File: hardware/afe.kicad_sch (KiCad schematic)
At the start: 6 parts, among them U2 LTC6813-1, U3 BQ76200PW

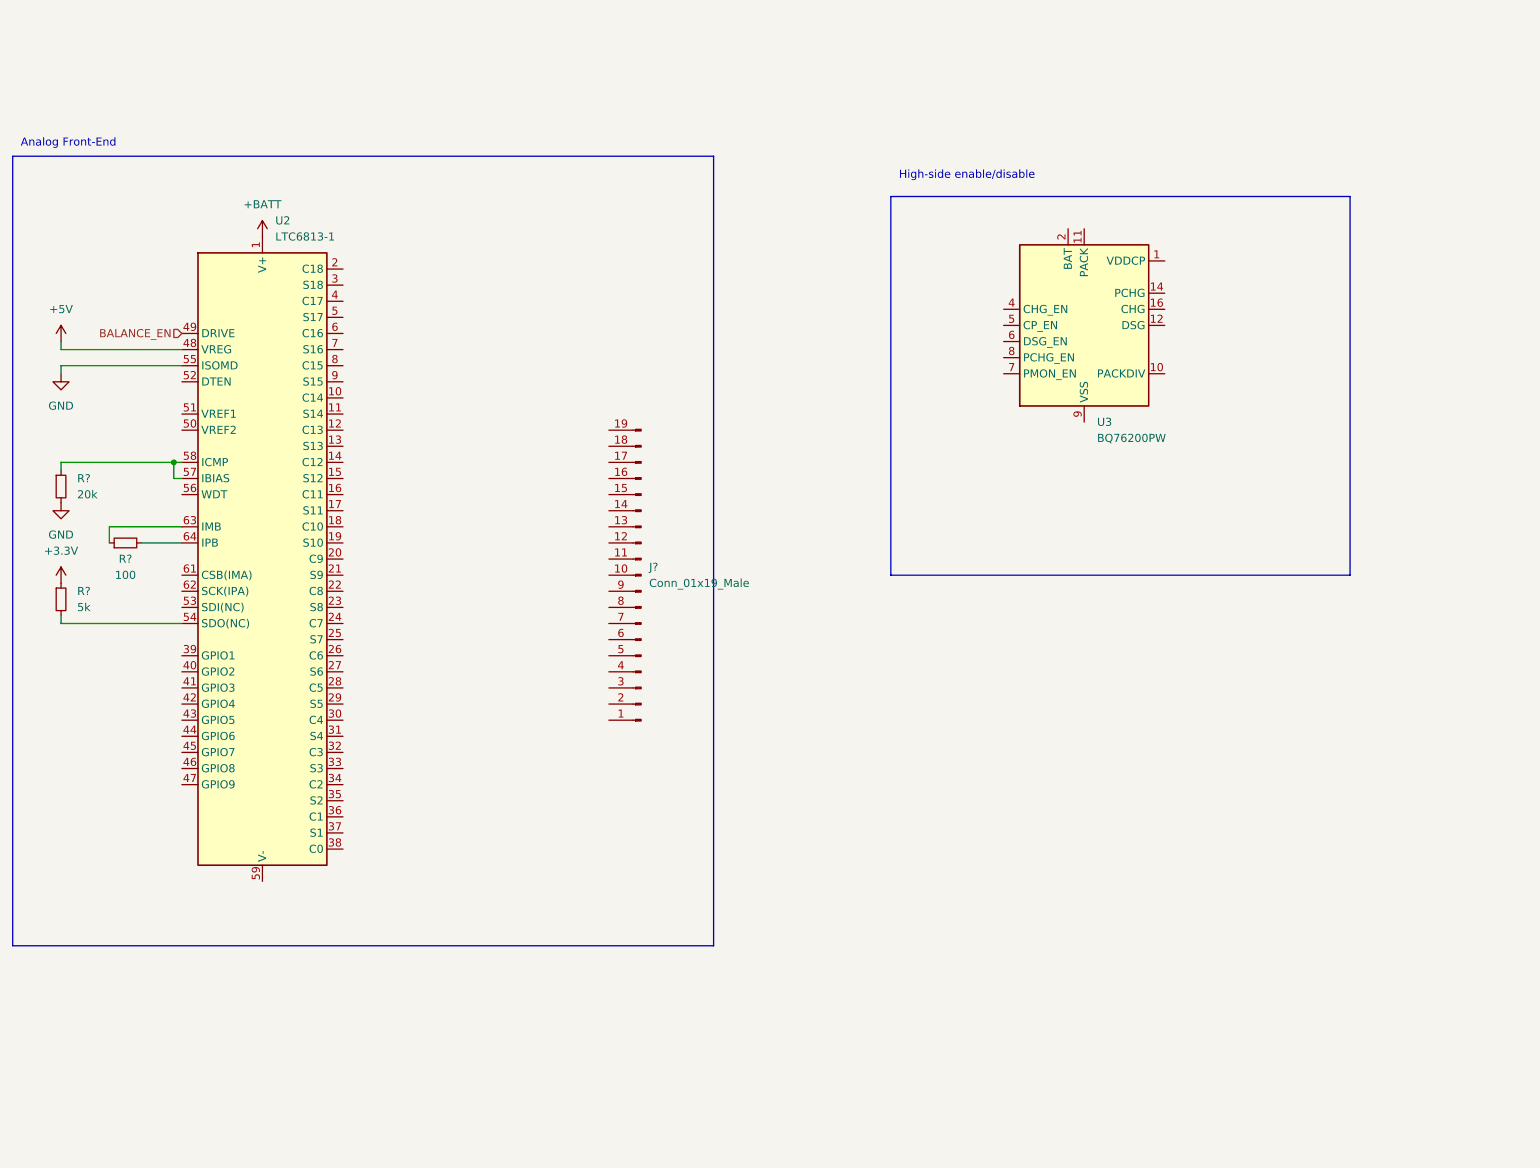
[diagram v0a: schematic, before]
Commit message: Balance frontend
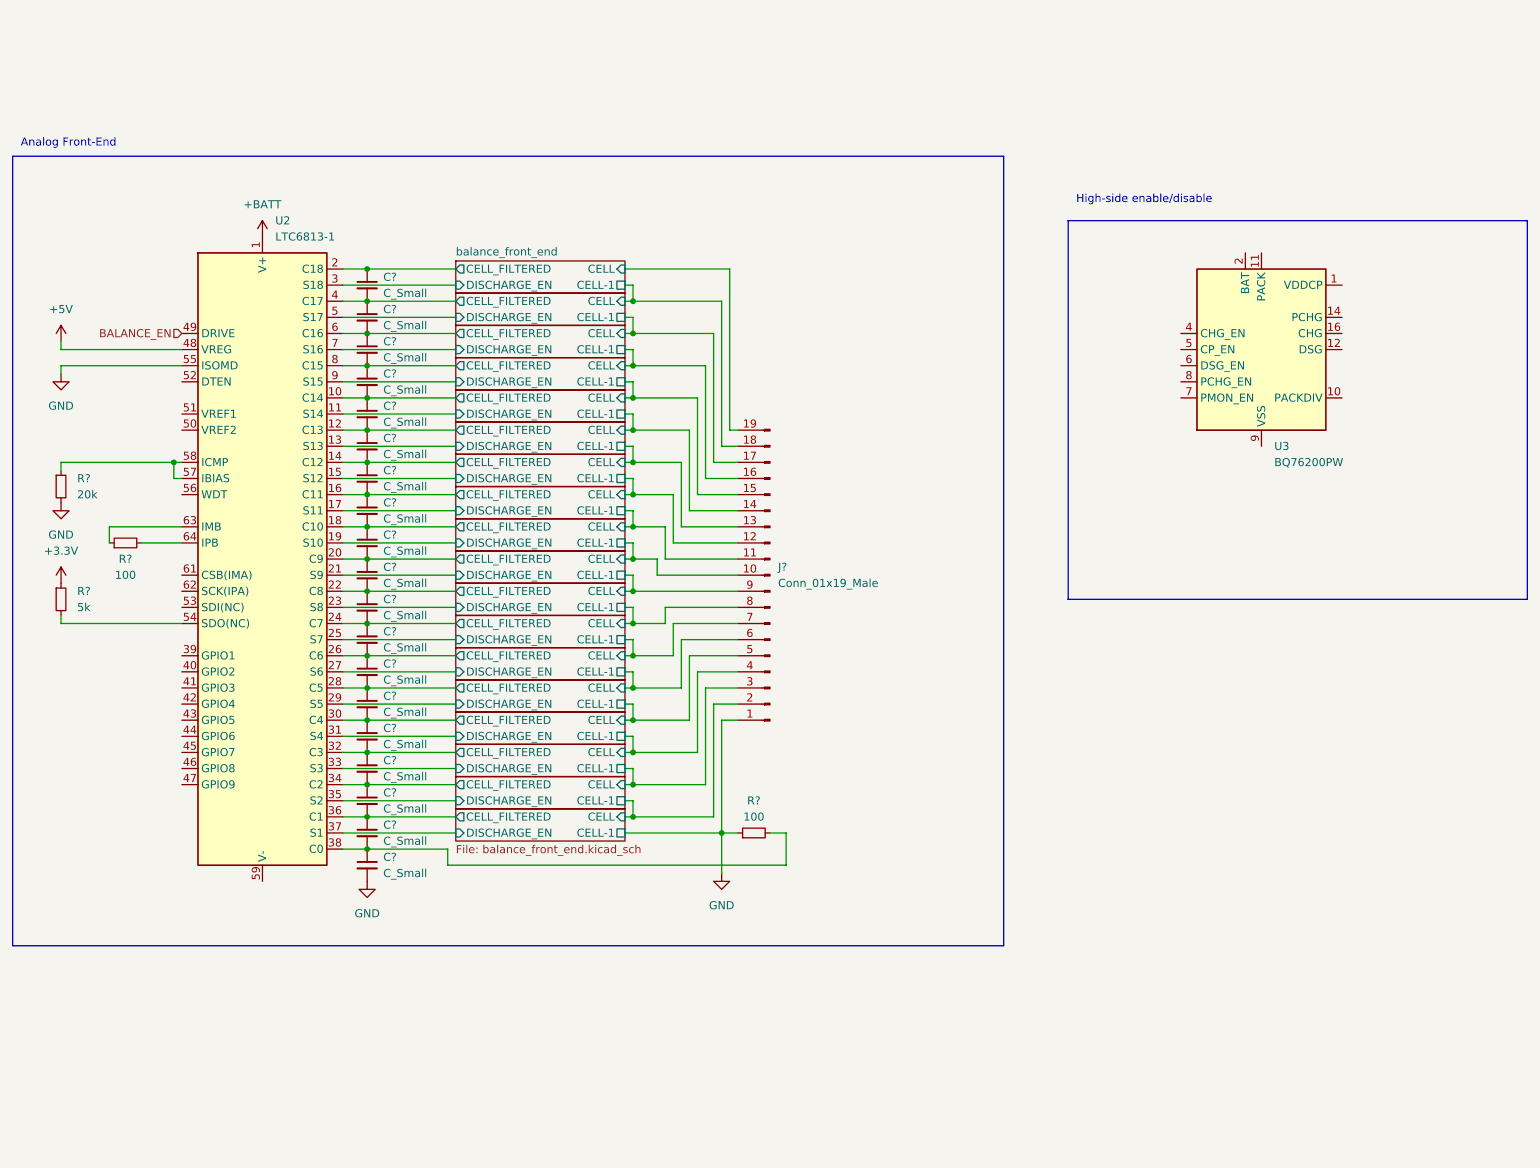
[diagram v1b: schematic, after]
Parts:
- added C? (x19): C_Small, symbol Device:C_Small
- added R?: 100, symbol Device:R_Small
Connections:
- net GND: now also J?.1 (Pin_1), C?.2, R?.1
- net balance_front_end6/CELL_FILTERED: now reaches U2.10 (C14)
- net balance_front_end6/CELL_FILTERED: now also C?.1, C?.2
- net balance_front_end6/DISCHARGE_EN: now reaches U2.11 (S14)
- net balance_front_end5/CELL_FILTERED: now reaches U2.12 (C13)
- net balance_front_end5/CELL_FILTERED: now also C?.1, C?.2
- net balance_front_end5/DISCHARGE_EN: now reaches U2.13 (S13)
- net balance_front_end4/CELL_FILTERED: now reaches U2.14 (C12)
- net balance_front_end4/CELL_FILTERED: now also C?.1, C?.2
- net balance_front_end4/DISCHARGE_EN: now reaches U2.15 (S12)
- net balance_front_end10/CELL_FILTERED: now reaches U2.16 (C11)
- net balance_front_end10/CELL_FILTERED: now also C?.1, C?.2
- net balance_front_end10/DISCHARGE_EN: now reaches U2.17 (S11)
- net balance_front_end9/CELL_FILTERED: now reaches U2.18 (C10)
- net balance_front_end9/CELL_FILTERED: now also C?.1, C?.2
- net balance_front_end9/DISCHARGE_EN: now reaches U2.19 (S10)
- net balance_front_end/CELL_FILTERED: now reaches U2.2 (C18)
- net balance_front_end/CELL_FILTERED: now also C?.1
- net balance_front_end7/CELL_FILTERED: now reaches U2.20 (C9)
- net balance_front_end7/CELL_FILTERED: now also C?.1, C?.2
- net balance_front_end7/DISCHARGE_EN: now reaches U2.21 (S9)
- net balance_front_end11/CELL_FILTERED: now reaches U2.22 (C8)
- net balance_front_end11/CELL_FILTERED: now also C?.1, C?.2
- net balance_front_end11/DISCHARGE_EN: now reaches U2.23 (S8)
- net balance_front_end12/CELL_FILTERED: now reaches U2.24 (C7)
- net balance_front_end12/CELL_FILTERED: now also C?.1, C?.2
- net balance_front_end12/DISCHARGE_EN: now reaches U2.25 (S7)
- net balance_front_end8/CELL_FILTERED: now reaches U2.26 (C6)
- net balance_front_end8/CELL_FILTERED: now also C?.1, C?.2
- net balance_front_end8/DISCHARGE_EN: now reaches U2.27 (S6)
- net balance_front_end13/CELL_FILTERED: now reaches U2.28 (C5)
- net balance_front_end13/CELL_FILTERED: now also C?.1, C?.2
- net balance_front_end13/DISCHARGE_EN: now reaches U2.29 (S5)
- net balance_front_end/DISCHARGE_EN: now reaches U2.3 (S18)
- net balance_front_end16/CELL_FILTERED: now reaches U2.30 (C4)
- net balance_front_end16/CELL_FILTERED: now also C?.1, C?.2
- net balance_front_end16/DISCHARGE_EN: now reaches U2.31 (S4)
- net balance_front_end14/CELL_FILTERED: now reaches U2.32 (C3)
- net balance_front_end14/CELL_FILTERED: now also C?.1, C?.2
- net balance_front_end14/DISCHARGE_EN: now reaches U2.33 (S3)
- net balance_front_end15/CELL_FILTERED: now reaches U2.34 (C2)
- net balance_front_end15/CELL_FILTERED: now also C?.1, C?.2
- net balance_front_end15/DISCHARGE_EN: now reaches U2.35 (S2)
- net balance_front_end17/CELL_FILTERED: now reaches U2.36 (C1)
- net balance_front_end17/CELL_FILTERED: now also C?.1, C?.2
- net balance_front_end17/DISCHARGE_EN: now reaches U2.37 (S1)
- net at U2.38 (C0): now also C?.1, C?.2, R?.2
- net balance_front_end1/CELL_FILTERED: now reaches U2.4 (C17)
- net balance_front_end1/CELL_FILTERED: now also C?.1, C?.2
- net balance_front_end1/DISCHARGE_EN: now reaches U2.5 (S17)
- net balance_front_end2/CELL_FILTERED: now reaches U2.6 (C16)
- net balance_front_end2/CELL_FILTERED: now also C?.1, C?.2
- net balance_front_end2/DISCHARGE_EN: now reaches U2.7 (S16)
- net balance_front_end3/CELL_FILTERED: now reaches U2.8 (C15)
- net balance_front_end3/CELL_FILTERED: now also C?.1, C?.2
- net balance_front_end3/DISCHARGE_EN: now reaches U2.9 (S15)
- net balance_front_end7/CELL: now reaches J?.10 (Pin_10)
- net balance_front_end10/CELL-1: now reaches J?.11 (Pin_11)
- net balance_front_end10/CELL: now reaches J?.12 (Pin_12)
- net balance_front_end4/CELL: now reaches J?.13 (Pin_13)
- net balance_front_end5/CELL: now reaches J?.14 (Pin_14)
- net balance_front_end3/CELL-1: now reaches J?.15 (Pin_15)
- net balance_front_end2/CELL-1: now reaches J?.16 (Pin_16)
- net balance_front_end1/CELL-1: now reaches J?.17 (Pin_17)
- net balance_front_end/CELL-1: now reaches J?.18 (Pin_18)
- net balance_front_end/CELL: now reaches J?.19 (Pin_19)
- net balance_front_end15/CELL-1: now reaches J?.2 (Pin_2)
- net balance_front_end14/CELL-1: now reaches J?.3 (Pin_3)
- net balance_front_end14/CELL: now reaches J?.4 (Pin_4)
- net balance_front_end13/CELL-1: now reaches J?.5 (Pin_5)
- net balance_front_end13/CELL: now reaches J?.6 (Pin_6)
- net balance_front_end12/CELL-1: now reaches J?.7 (Pin_7)
- net balance_front_end11/CELL-1: now reaches J?.8 (Pin_8)
- net balance_front_end11/CELL: now reaches J?.9 (Pin_9)
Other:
- added sheet balance_front_end (balance_front_end.kicad_sch)
- added sheet balance_front_end1 (balance_front_end.kicad_sch)
- added sheet balance_front_end10 (balance_front_end.kicad_sch)
- added sheet balance_front_end11 (balance_front_end.kicad_sch)
- added sheet balance_front_end12 (balance_front_end.kicad_sch)
- added sheet balance_front_end13 (balance_front_end.kicad_sch)
- added sheet balance_front_end14 (balance_front_end.kicad_sch)
- added sheet balance_front_end15 (balance_front_end.kicad_sch)
- added sheet balance_front_end16 (balance_front_end.kicad_sch)
- added sheet balance_front_end17 (balance_front_end.kicad_sch)
- added sheet balance_front_end2 (balance_front_end.kicad_sch)
- added sheet balance_front_end3 (balance_front_end.kicad_sch)
- added sheet balance_front_end4 (balance_front_end.kicad_sch)
- added sheet balance_front_end5 (balance_front_end.kicad_sch)
- added sheet balance_front_end6 (balance_front_end.kicad_sch)
- added sheet balance_front_end7 (balance_front_end.kicad_sch)
- added sheet balance_front_end8 (balance_front_end.kicad_sch)
- added sheet balance_front_end9 (balance_front_end.kicad_sch)
- moved on the sheet: J?, U3

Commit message: Analog front end daisy chain
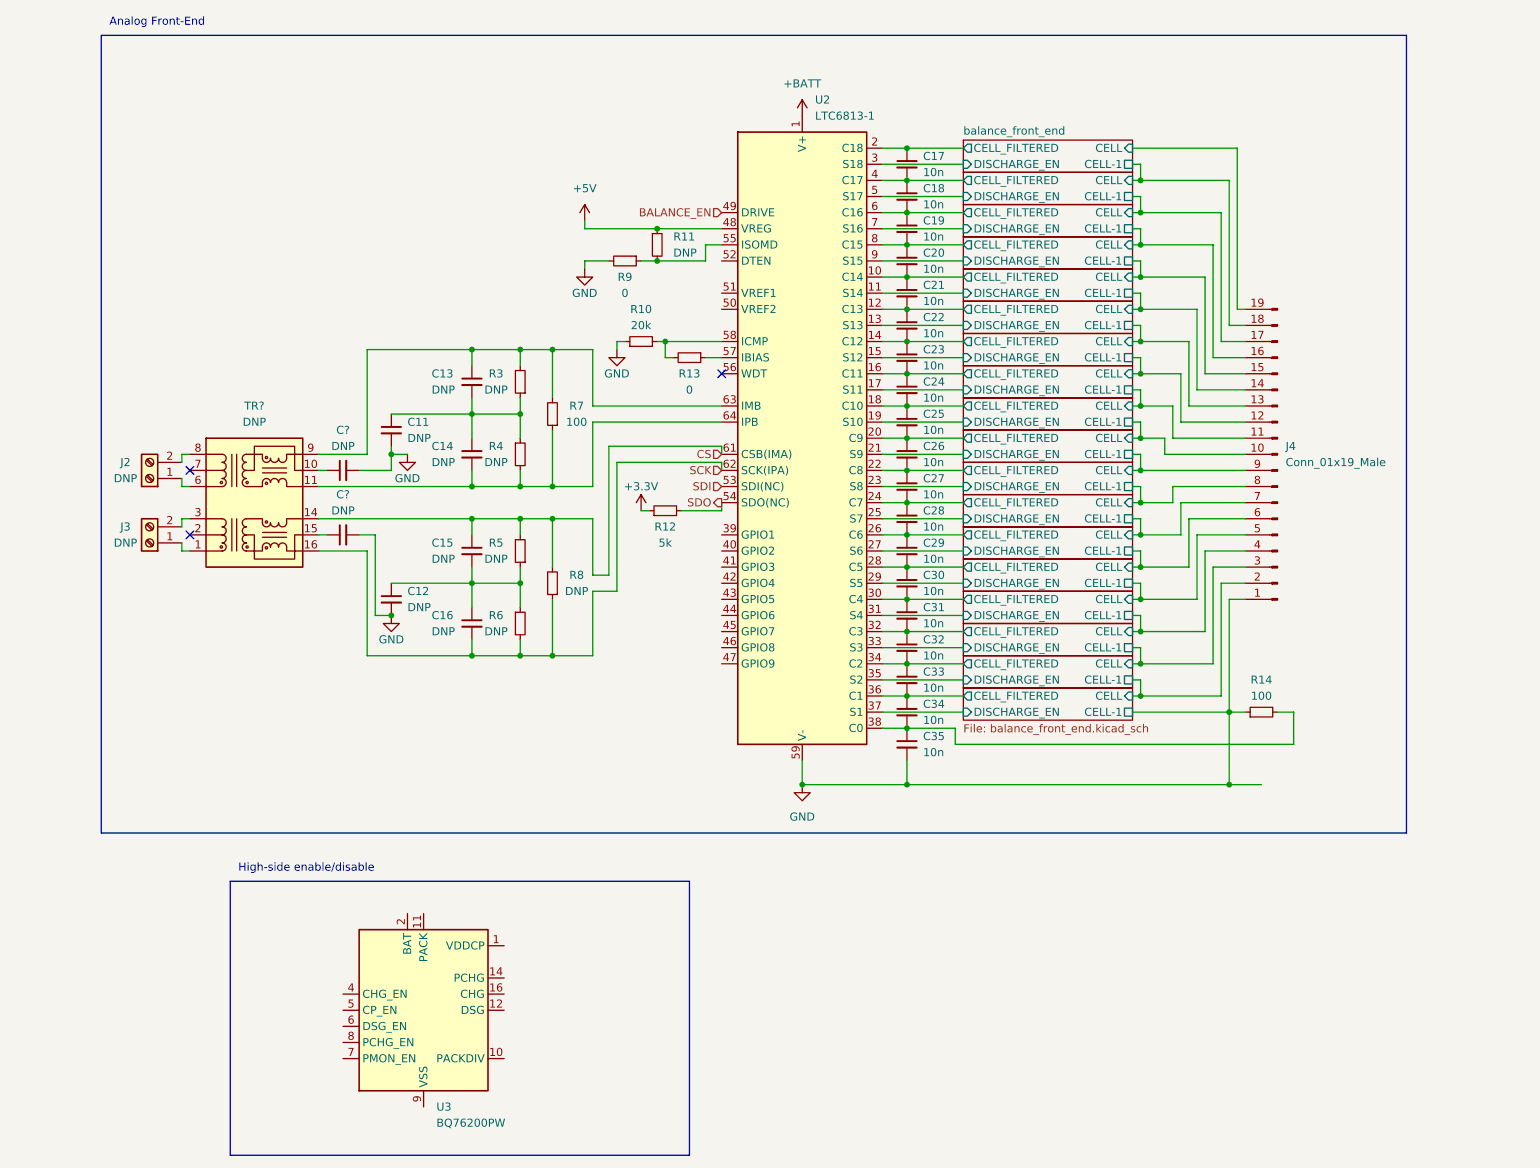
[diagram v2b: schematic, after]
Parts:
- added C11, C12, C13, C14, C15, C16, C? (x2): DNP, symbol Device:C_Small
- added J2, J3: DNP, symbol Connector:Screw_Terminal_01x02
- added R11, R3, R4, R5, R6, R8: DNP, symbol Device:R_Small
- added R13, R9: 0, symbol Device:R_Small
- added TR?: DNP, Transformer_SMD:Transformer_Ethernet_Bourns_PT61017PEL, symbol vesc-bms:HM2102NLT
- C17, C18, C19, C20, C21, C22, C23, C24, C25, C26, C27, C28, C29, C30, C31, C32, C33, C34, C35: renamed from C?; value C_Small -> 10n
- gave numbers to parts that had none: 5
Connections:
- net +5V: now also R11.1
- net GND: now also R10.1, U2.59 (V-), U2.60 (V-), C11.2, C12.2, C?.2, C?.2, R9.2; no longer R10.2, U2.55 (ISOMD)
- net SDI: now reaches U2.53 (SDI(NC))
- net SDO: now reaches R12.2, U2.54 (SDO(NC))
- net CS: now reaches U2.61 (CSB(IMA))
- net CS: now also C15.1, R5.2, R8.2, TR?.14 (TX-)
- net SCK: now reaches U2.62 (SCK(IPA))
- net SCK: now also C16.2, R6.2, R8.1, TR?.16 (TX+)
- net at U2.63 (IMB): now also R7.2, C13.1, R3.2, TR?.9 (RX-); no longer R7.1
- net at U2.64 (IPB): now also R7.1, C14.2, R4.2, TR?.11 (RX+); no longer R7.2
- new net: C?.1, TR?.10 (C_RX)
- new net: R11.2, R9.1, U2.55 (ISOMD)
- new net: C12.1, C15.2, C16.1, R5.1, R6.1
- new net: R13.1, U2.57 (IBIAS)
- new net: R10.2, R13.2, U2.58 (ICMP)
- new net: J3.1 (Pin_1), TR?.1 (TD+)
- new net: C?.1, TR?.15 (C_TX)
- new net: J3.2 (Pin_2), TR?.3 (TD-)
- new net: J2.1 (Pin_1), TR?.6 (RD+)
- new net: J2.2 (Pin_2), TR?.8 (RD-)
- new net: C11.1, C13.2, C14.1, R3.1, R4.1
- no-connect marks 0 -> 3
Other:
- moved on the sheet: C17, C18, C19, C20, C21, C22, C23, C24, C25, C26, C27, C28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
